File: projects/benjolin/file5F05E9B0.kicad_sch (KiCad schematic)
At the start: 15 parts, among them J2 power-barrel-jack, U1 78L09, U2 79L09

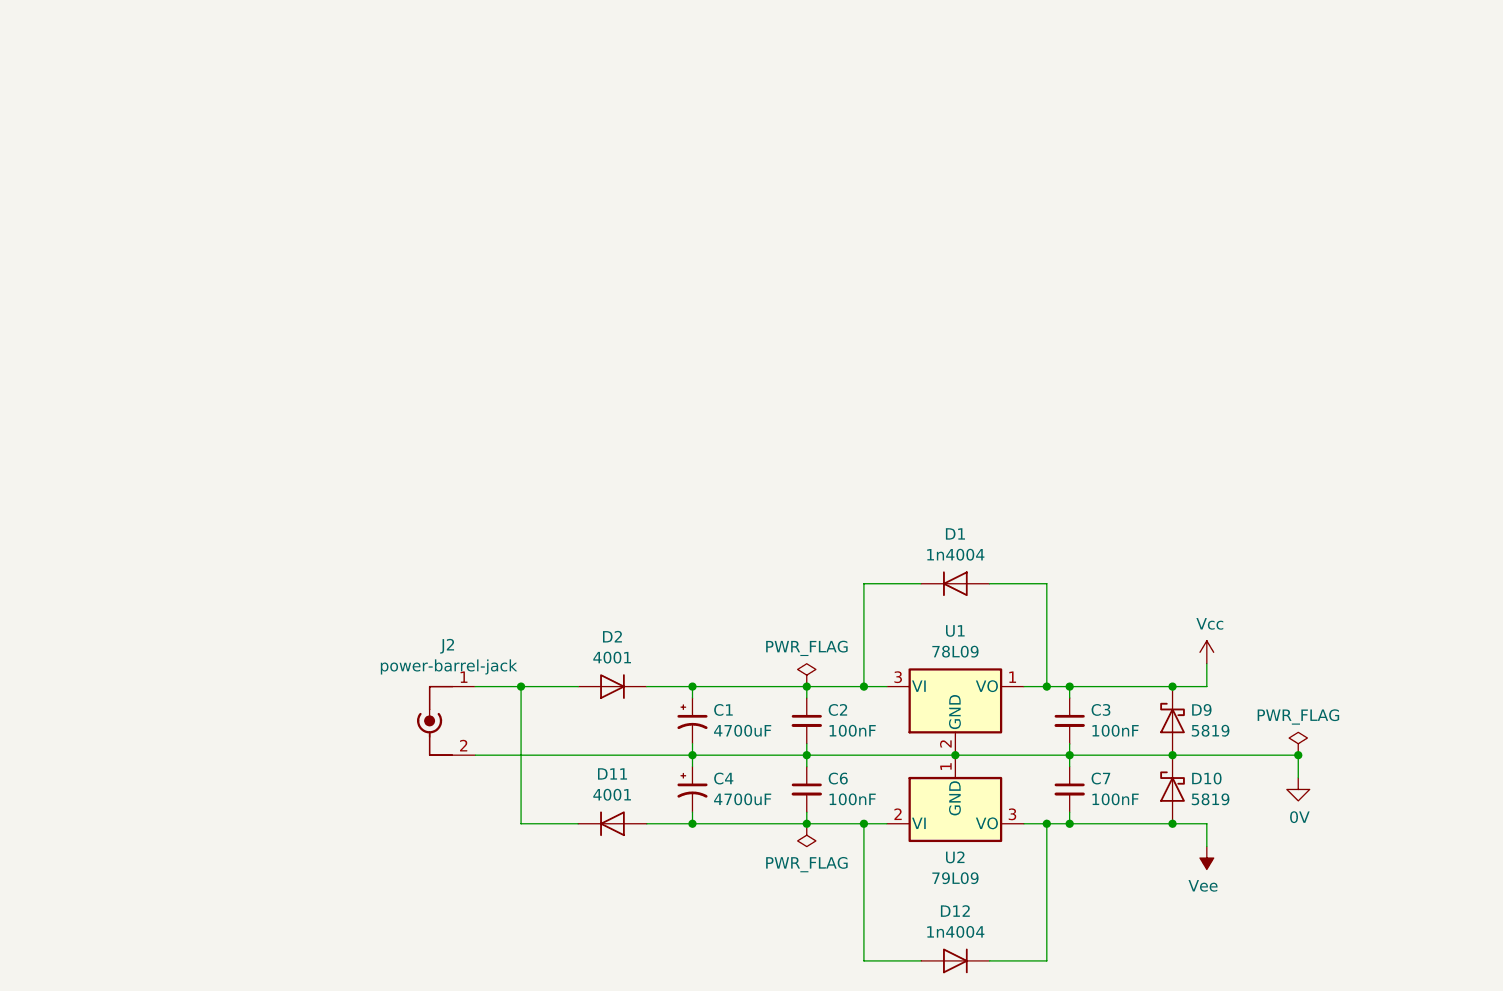
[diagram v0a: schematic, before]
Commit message: it's a dual benjolin
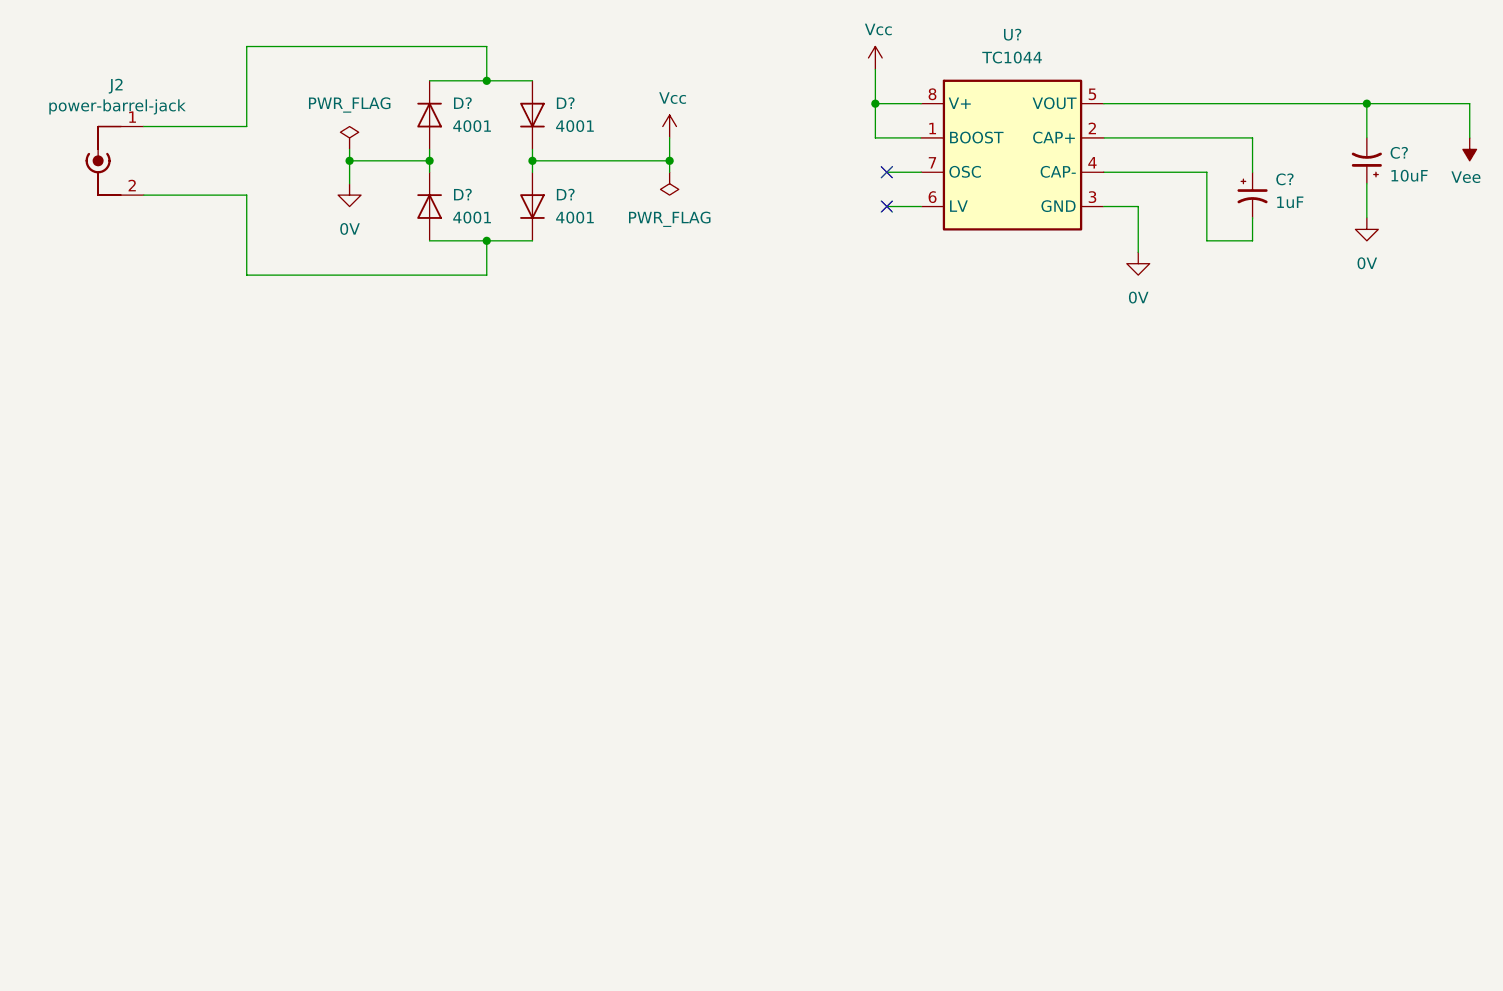
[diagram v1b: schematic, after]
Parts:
- removed C1, C4: 4700uF, 00-Mine:capacitor-7.5mmLS, symbol 00-cool_stuff:cap_polarized_small
- removed C2, C3, C6, C7: 100nF, 00-Mine:capacitor-TH-2.54mm, symbol 00-cool_stuff:cap_small
- removed D1, D12: 1n4004, 00-Mine:diode-TH, symbol 00-cool_stuff:diode
- removed D10, D9: 5819, 00-Mine:diode-TH, symbol power1-rescue:schottky-diode-00-cool_stuff
- removed D11, D2: 4001, 00-Mine:diode-TH, symbol 00-cool_stuff:diode
- removed U1: 78L09, 00-Mine:TO-92_HandSolder, symbol 00-cool_stuff:78L0X
- removed U2: 79L09, 00-Mine:TO-92_HandSolder, symbol 00-cool_stuff:79L0X
- added C?: 1uF, symbol 00-cool_stuff:cap_polarized_small
- added C?: 10uF, symbol 00-cool_stuff:cap_polarized_small
- added D? (x4): 4001, 00-Mine:diode-TH, symbol 00-cool_stuff:diode
- added U?: TC1044, symbol 00-cool_stuff:TC1044
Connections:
- net GND: now also C?.1, D?.1 (K), D?.2 (A), U?.3 (GND); no longer J2.2 (Ext)
- net Vcc: now also D?.1 (K), D?.2 (A), U?.1 (BOOST), U?.8 (V+)
- net Vee: now also C?.2, U?.5 (VOUT)
- net at J2.1 (In): now also D?.1 (K), D?.2 (A)
- new net: D?.1 (K), D?.2 (A), J2.2 (Ext)
- new net: C?.1, U?.2 (CAP+)
- new net: C?.2, U?.4 (CAP-)
- no-connect marks 0 -> 2
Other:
- moved on the sheet: J2
